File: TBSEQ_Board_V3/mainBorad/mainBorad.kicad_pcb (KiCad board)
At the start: 2 copper layers, 258 parts, among them IC1 NJM2125F-TE1_DIP8, IC12 4066, IC2 NJM2125F-TE1_DIP8, IC4 NJM2125F-TE1, IC5 NJM2125F-TE1_DIP8, J1 Conn_01x08, J10 Conn_01x05, J11 Conn_01x05, J12 Conn_01x02, J13 Conn_01x01_Pin, J14 Conn_01x05, J2 Conn_01x05_Pin, J3 Conn_01x02_Pin, J4 Conn_01x03, J5 Conn_01x03, J6 MJ-462, J7 Conn_01x03_Pin, J8 Conn_01x02_Pin, J9 Conn_01x01_Pin, Q1 NPN, Q10 PNP, Q11 NPN, Q12 HN1C01FU-GR,LF, Q13 NPN, Q14 NPN, Q15 NPN, Q16 NPN, Q17 NPN, Q18 NPN, Q19 NPN, Q2 PNP, Q20 NPN, Q21 HN1C01FU-GR,LF, Q22 HN1C01FU-GR,LF, Q23 NPN, Q24 NPN, Q25 NPN, Q26 HN1C01FU-GR,LF, Q27 PNP, Q28 NJFET, Q29 NPN, Q30 NPN, Q35 NPN, Q36 PNP, Q37 NPN, Q38 PNP, Q39 NJFET, Q40 NPN, Q41 NPN, Q8 PNP, Q9 PNP, SW1 2MS1T1B4VS2QES, U1 LM13700

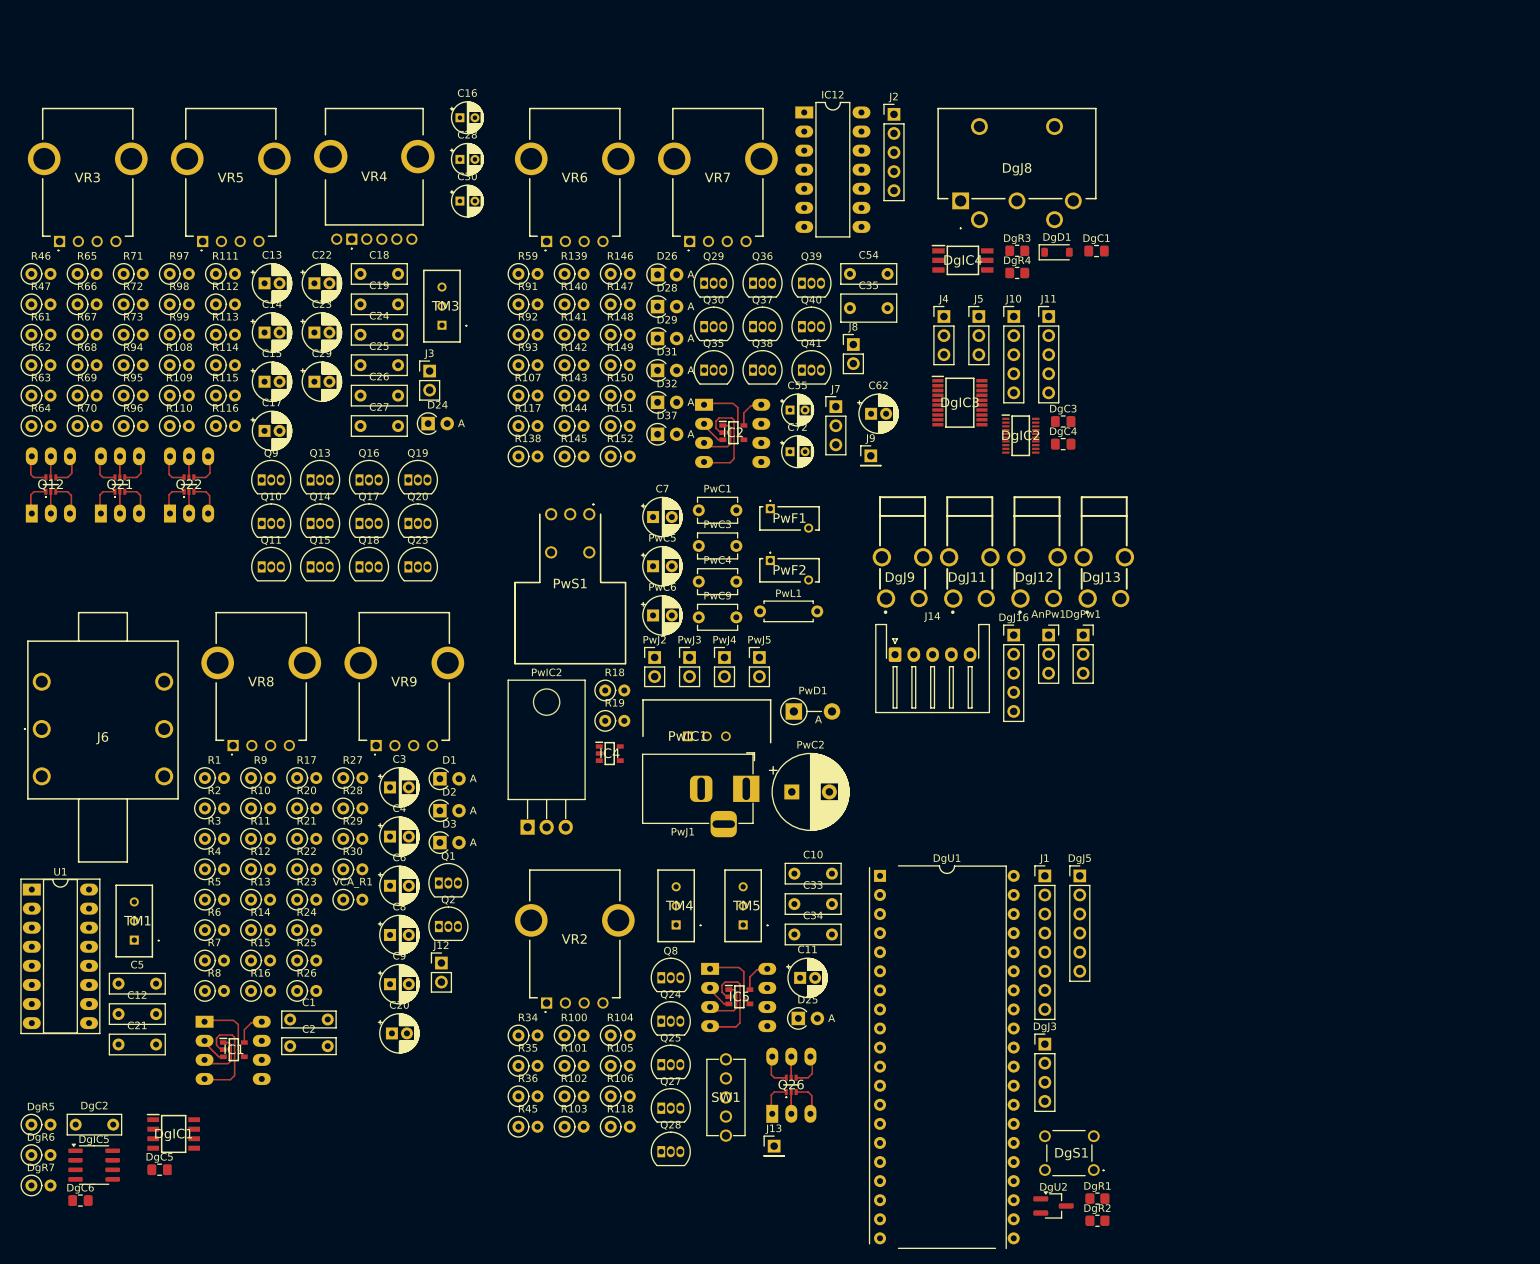
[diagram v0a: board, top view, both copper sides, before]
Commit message: V3Board
アートワーク中
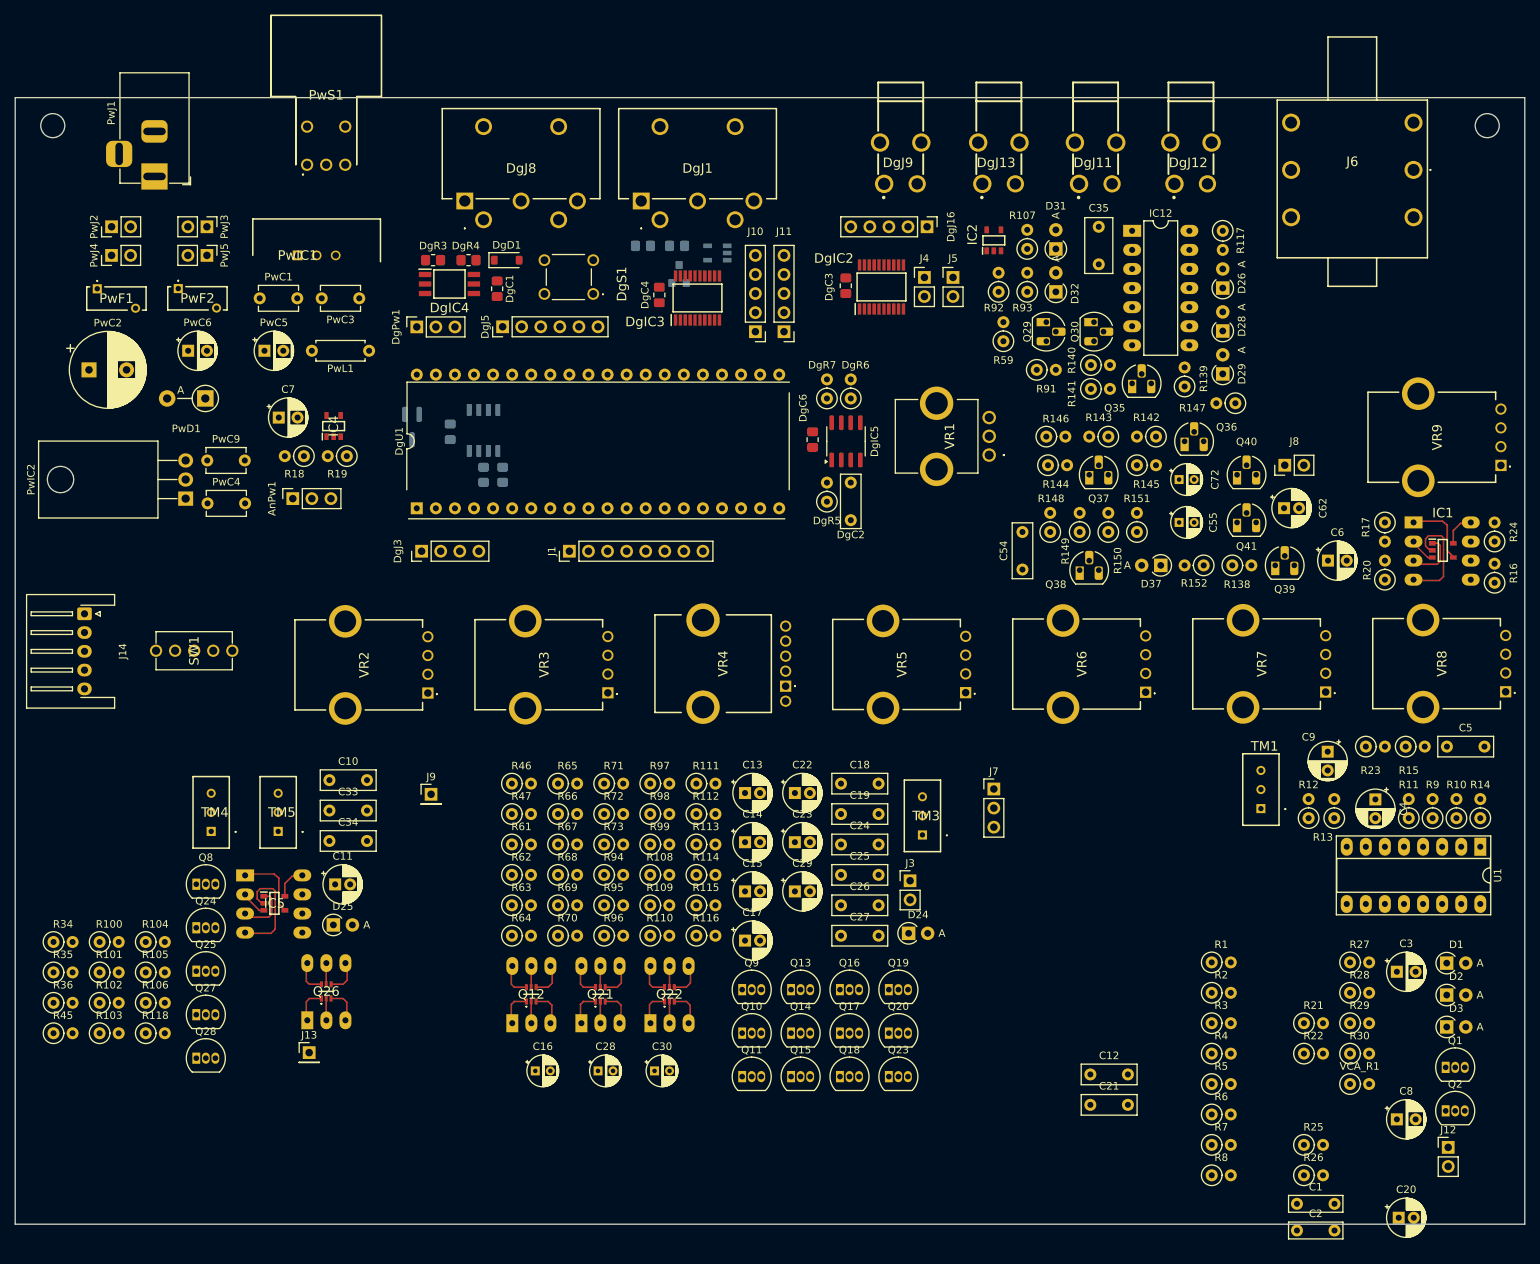
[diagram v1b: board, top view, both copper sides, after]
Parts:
- removed J2: Conn_01x05_Pin, Connector_PinHeader_2.54mm:PinHeader_1x05_P2.54mm_Vertical
- added DgJ1: KDJ03-5 MIDIOUT, SamacSys_Parts:KDJ035, F.Cu at (107.4, 34.0)
- added DgR8: 220, Resistor_SMD:R_0805_2012Metric_Pad1.20x1.40mm_HandSolder, B.Cu at (107.6, 40.0)
- added DgR9: 220, Resistor_SMD:R_0805_2012Metric_Pad1.20x1.40mm_HandSolder, B.Cu at (112.1, 40.0)
- added IC3: 74AHC1G04W5-7, SamacSys_Parts:SOT95P285X140-5N, B.Cu at (117.5, 41.0)
- added Q4: 2SC3325-Y, SamacSys_Parts:2SC3325YLF, B.Cu at (112.4, 44.2)
- added VR1: RK09D117000B, SamacSys_Parts:RK09D117000B, F.Cu at (153.7, 67.9)
- DgC5, DgIC1, DgR1, DgR2, DgU2: moved to B.Cu
- DgIC2: value TC74VHC541FK -> 74VHC541FT; footprint SamacSys_Parts:SOP50P400X100-20N -> SamacSys_Parts:SOP65P640X120-20N
- DgIC3: value 74LVC541APW -> 74VHC541FT; footprint SamacSys_Parts:SOP65P640X110-20N -> SamacSys_Parts:SOP65P640X120-20N
- DgJ11: value MJ-8435 -> MJ-8435 CV OUT
- DgJ12: value MJ-8435 -> MJ-8435 GATE OUT
- DgJ13: value MJ-8435 -> MJ-8435 SYNC OUT
- DgJ8: value KDJ03-5 -> KDJ03-5 MIDIIN
- DgJ9: value MJ-8435 -> MJ-8435 SYNC IN
- IC2: value NJM2125F-TE1_DIP8 -> NJM2125F-TE1; footprint SamacSys_Parts:NJM2125F-SOT95&DIP8 -> SamacSys_Parts:SOT95P280X130-5N
- J4, J5: value Conn_01x03 -> Conn_01x02; footprint Connector_PinHeader_2.54mm:PinHeader_1x03_P2.54mm_Vertical -> Connector_PinHeader_2.54mm:PinHeader_1x02_P2.54mm_Vertical
- Q29, Q30, Q35, Q36, Q37, Q38, Q39, Q40, Q41: footprint Package_TO_SOT_THT:TO-92_Inline -> Package_TO_SOT_THT:TO-92_HandSolder
- moved J6 197.2 mm to (210.2, 29.9), turned to 180 degrees
- moved U1 192.9 mm to (219.1, 120.0), turned to -90 degrees
- moved C5 179.7 mm to (214.6, 106.7)
- moved R16 174.3 mm to (221.0, 84.9), turned to 90 degrees
- moved IC1 174.2 mm to (214.1, 80.6)
- moved VR8 169.6 mm to (222.5, 99.4), turned to 90 degrees
- moved R24 167.6 mm to (221.0, 79.4), turned to 90 degrees
- moved R14 164.4 mm to (219.1, 116.2), turned to 90 degrees
- moved R10 160.5 mm to (215.9, 116.2), turned to 90 degrees
- moved R9 157.4 mm to (212.7, 116.2), turned to 90 degrees
- moved R15 156.4 mm to (209.1, 106.7)
- moved VR9 154.3 mm to (221.8, 69.2), turned to 90 degrees
- moved R11 154.2 mm to (209.6, 116.2), turned to 90 degrees
- moved TM1 151.0 mm to (189.9, 114.9)
- moved DgR7 149.0 mm to (132.1, 60.3), turned to 90 degrees
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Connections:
- DgIC2 pad 13: Net-(DgIC2-Y6) -> D+5V_MIDITX
- DgIC2 pad 7: Net-(DgIC2-A6) -> D+3.3V_MIDITX
- DgJ3 pad 1: Net-(DgJ3-Pin_1) -> D+3.3V_MIDITX
- DgU1 pad 1: Net-(DgJ3-Pin_1) -> D+3.3V_MIDITX
- IC2 pad 1: A+VCO_CV -> A+CV
- IC2 pad 2: Net-(IC2--INPUT) -> GNDA
- IC2 pad 3: A+CV -> Net-(IC2--INPUT)
- IC2 pad 4: GNDA -> A+VCO_CV
- IC2 pad 5: unconnected-(IC2-NC-Pad5) -> A+12V
- J14 pad 4: A+TEMPO -> unconnected-(J14-Pin_4-Pad4)
- J4 pad 1: Net-(DgIC2-A6) -> Net-(DgIC2-A7)
- J4 pad 2: Net-(DgIC2-A7) -> Net-(DgIC2-A8)
- J5 pad 1: Net-(DgIC2-Y6) -> Net-(DgIC2-Y7)
- J5 pad 2: Net-(DgIC2-Y7) -> Net-(DgIC2-Y8)
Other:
- board outline added: 201 x 150 mm
